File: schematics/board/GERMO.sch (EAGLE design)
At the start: 28 parts

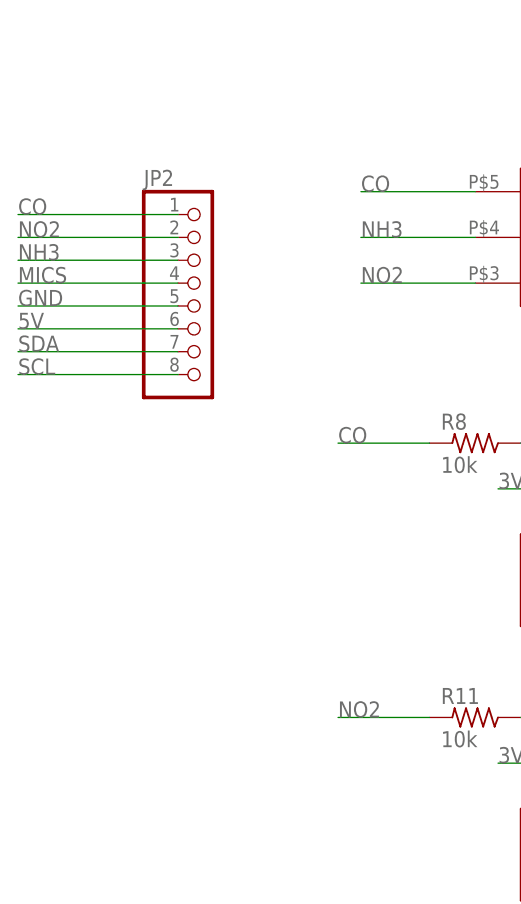
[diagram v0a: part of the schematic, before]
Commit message: сч мипэхъ\
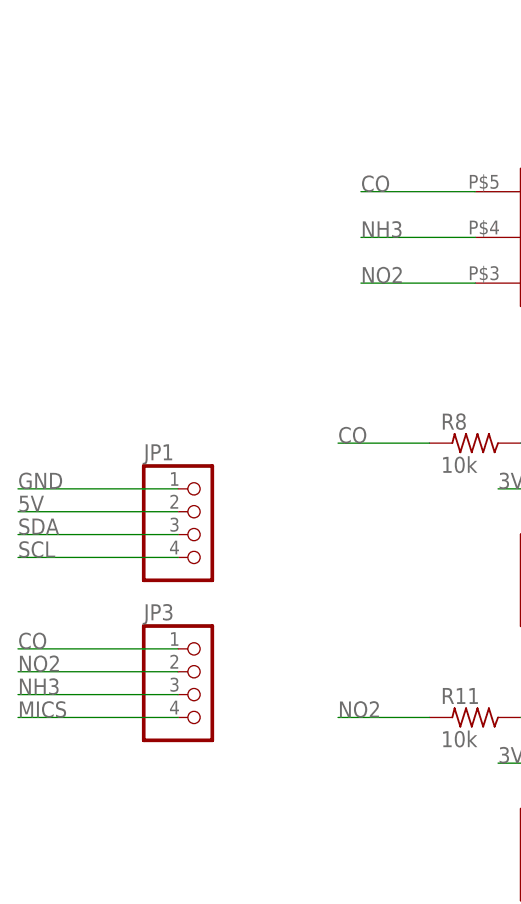
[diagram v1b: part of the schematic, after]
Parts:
- removed JP2: (no value), pinhead:PINHD-1X8
- added JP1, JP3: (no value), pinhead:PINHD-1X4
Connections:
- net 5V: now also JP1.2; no longer JP2.6
- net CO: now also JP3.1; no longer JP2.1
- net GND: now also JP1.1; no longer JP2.5
- net MICS: now also JP3.4; no longer JP2.4
- net NH3: now also JP3.3; no longer JP2.3
- net NO2: now also JP3.2; no longer JP2.2
- net SCL: now also JP1.4; no longer JP2.8
- net SDA: now also JP1.3; no longer JP2.7
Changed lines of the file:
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@@
 <?xml version="1.0" encoding="utf-8"?>
 <!DOCTYPE eagle SYSTEM "eagle.dtd">
-<eagle version="9.4.2">
+<eagle version="9.6.2">
 <drawing>
 <settings>
-<setting alwaysvectorfont="yes"/>
+<setting alwaysvectorfont="no"/>
 <setting verticaltext="up"/>
 </settings>
@@
 </classes>
 <parts>
-<part name="JP2" library="pinhead" library_urn="urn:adsk.eagle:library:325" deviceset="PINHD-1X8" device="" package3d_urn="urn:adsk.eagle:package:22409/2"/>
 <part name="BME280" library="UNKNOWN-2024" deviceset="BME280" device="BME280-PINS-ONLY"/>
 <part name="MICS-6814" library="CanCubeSat" deviceset="MICS-6814" device=""/>
@@
 <part name="U$11" library="UNKNOWN-2024" deviceset="CONNECT_3" device=""/>
 <part name="U$12" library="UNKNOWN-2024" deviceset="CONNECT_3" device=""/>
+<part name="JP1" library="pinhead" library_urn="urn:adsk.eagle:library:325" deviceset="PINHD-1X4" device="" package3d_urn="urn:adsk.eagle:package:22407/2"/>
+<part name="JP3" library="pinhead" library_urn="urn:adsk.eagle:library:325" deviceset="PINHD-1X4" device="" package3d_urn="urn:adsk.eagle:package:22407/2"/>
 </parts>
 <sheets>
@@
 </plain>
 <instances>
-<instance part="JP2" gate="A" x="-101.6" y="43.18" smashed="yes">
-<attribute name="NAME" x="-107.95" y="56.515" size="1.778" layer="95"/>
-<attribute name="VALUE" x="-107.95" y="30.48" size="1.778" layer="96"/>
-</instance>
 <instance part="BME280" gate="G$1" x="86.36" y="20.32" smashed="yes">
 <attribute name="NAME" x="82.296" y="26.416" size="1.27" layer="95"/>
@@
 <instance part="U$12" gate="G$1" x="30.48" y="-12.7" smashed="yes" rot="R270">
 <attribute name="NAME" x="38.1" y="-12.7" size="1.778" layer="95" rot="R270"/>
+</instance>
+<instance part="JP1" gate="A" x="-101.6" y="17.78" smashed="yes">
+<attribute name="NAME" x="-107.95" y="26.035" size="1.778" layer="95"/>
+<attribute name="VALUE" x="-107.95" y="10.16" size="1.778" layer="96"/>
+</instance>
+<instance part="JP3" gate="A" x="-101.6" y="0" smashed="yes">
+<attribute name="NAME" x="-107.95" y="8.255" size="1.778" layer="95"/>
+<attribute name="VALUE" x="-107.95" y="-7.62" size="1.778" layer="96"/>
 </instance>
 </instances>
@@
 <net name="GND" class="0">
 <segment>
-<wire x1="-104.14" y1="43.18" x2="-121.92" y2="43.18" width="0.1524" layer="91"/>
-<label x="-121.92" y="43.18" size="1.778" layer="95"/>
-<pinref part="JP2" gate="A" pin="5"/>
-</segment>
-<segment>
 <wire x1="73.66" y1="17.78" x2="60.96" y2="17.78" width="0.1524" layer="91"/>
 <label x="60.96" y="17.78" size="1.778" layer="95"/>
@@
 <label x="63.5" y="48.26" size="1.778" layer="95"/>
 </segment>
+<segment>
+<wire x1="-104.14" y1="22.86" x2="-121.92" y2="22.86" width="0.1524" layer="91"/>
+<label x="-121.92" y="22.86" size="1.778" layer="95"/>
+<pinref part="JP1" gate="A" pin="1"/>
+</segment>
 </net>
 <net name="5V" class="0">
-<segment>
-<wire x1="-104.14" y1="40.64" x2="-121.92" y2="40.64" width="0.1524" layer="91"/>
-<label x="-121.92" y="40.64" size="1.778" layer="95"/>
-<pinref part="JP2" gate="A" pin="6"/>
-</segment>
 <segment>
 <pinref part="BME280" gate="G$1" pin="VIN"/>
@@
 <label x="83.82" y="58.42" size="1.778" layer="95"/>
 </segment>
+<segment>
+<wire x1="-104.14" y1="20.32" x2="-121.92" y2="20.32" width="0.1524" layer="91"/>
+<label x="-121.92" y="20.32" size="1.778" layer="95"/>
+<pinref part="JP1" gate="A" pin="2"/>
+</segment>
 </net>
 <net name="NO2" class="0">
-<segment>
-<wire x1="-121.92" y1="50.8" x2="-104.14" y2="50.8" width="0.1524" layer="91"/>
-<label x="-121.92" y="50.8" size="1.778" layer="95"/>
-<pinref part="JP2" gate="A" pin="2"/>
-</segment>
 <segment>
 <pinref part="MICS-6814" gate="G$1" pin="NO2"/>
@@
 <label x="-86.36" y="-2.54" size="1.778" layer="95"/>
 </segment>
+<segment>
+<wire x1="-121.92" y1="2.54" x2="-104.14" y2="2.54" width="0.1524" layer="91"/>
+<label x="-121.92" y="2.54" size="1.778" layer="95"/>
+<pinref part="JP3" gate="A" pin="2"/>
+</segment>
 </net>
 <net name="NH3" class="0">
-<segment>
-<wire x1="-104.14" y1="48.26" x2="-121.92" y2="48.26" width="0.1524" layer="91"/>
-<label x="-121.92" y="48.26" size="1.778" layer="95"/>
-<pinref part="JP2" gate="A" pin="3"/>
-</segment>
 <segment>
 <pinref part="MICS-6814" gate="G$1" pin="NH3"/>
@@
 <label x="-12.7" y="27.94" size="1.778" layer="95"/>
 </segment>
+<segment>
+<wire x1="-104.14" y1="0" x2="-121.92" y2="0" width="0.1524" layer="91"/>
+<label x="-121.92" y="0" size="1.778" layer="95"/>
+<pinref part="JP3" gate="A" pin="3"/>
+</segment>
 </net>
 <net name="MICS" class="0">
-<segment>
-<wire x1="-121.92" y1="45.72" x2="-104.14" y2="45.72" width="0.1524" layer="91"/>
-<label x="-121.92" y="45.72" size="1.778" layer="95"/>
-<pinref part="JP2" gate="A" pin="4"/>
-</segment>
 <segment>
 <wire x1="17.78" y1="48.26" x2="5.08" y2="48.26" width="0.1524" layer="91"/>
@@
 <label x="-12.7" y="-2.54" size="1.778" layer="95"/>
 </segment>
+<segment>
+<wire x1="-121.92" y1="-2.54" x2="-104.14" y2="-2.54" width="0.1524" layer="91"/>
+<label x="-121.92" y="-2.54" size="1.778" layer="95"/>
+<pinref part="JP3" gate="A" pin="4"/>
+</segment>
 </net>
 <net name="SDA" class="0">
-<segment>
-<wire x1="-104.14" y1="38.1" x2="-121.92" y2="38.1" width="0.1524" layer="91"/>
-<label x="-121.92" y="38.1" size="1.778" layer="95"/>
-<pinref part="JP2" gate="A" pin="7"/>
-</segment>
 <segment>
 <wire x1="99.06" y1="17.78" x2="114.3" y2="17.78" width="0.1524" layer="91"/>
@@
 <label x="83.82" y="50.8" size="1.778" layer="95"/>
 </segment>
+<segment>
+<wire x1="-104.14" y1="17.78" x2="-121.92" y2="17.78" width="0.1524" layer="91"/>
+<label x="-121.92" y="17.78" size="1.778" layer="95"/>
+<pinref part="JP1" gate="A" pin="3"/>
+</segment>
 </net>
 <net name="SCL" class="0">
-<segment>
-<wire x1="-104.14" y1="35.56" x2="-121.92" y2="35.56" width="0.1524" layer="91"/>
-<label x="-121.92" y="35.56" size="1.778" layer="95"/>
-<pinref part="JP2" gate="A" pin="8"/>
-</segment>
 <segment>
 <wire x1="99.06" y1="22.86" x2="114.3" y2="22.86" width="0.1524" layer="91"/>
@@
 <label x="83.82" y="53.34" size="1.778" layer="95"/>
 </segment>
+<segment>
+<wire x1="-104.14" y1="15.24" x2="-121.92" y2="15.24" width="0.1524" layer="91"/>
+<label x="-121.92" y="15.24" size="1.778" layer="95"/>
+<pinref part="JP1" gate="A" pin="4"/>
+</segment>
 </net>
 <net name="CO" class="0">
@@
 </segment>
 <segment>
-<wire x1="-104.14" y1="53.34" x2="-121.92" y2="53.34" width="0.1524" layer="91"/>
-<label x="-121.92" y="53.34" size="1.778" layer="95"/>
-<pinref part="JP2" gate="A" pin="1"/>
-</segment>
-<segment>
 <pinref part="R8" gate="G$1" pin="2"/>
 <wire x1="-76.2" y1="27.94" x2="-86.36" y2="27.94" width="0.1524" layer="91"/>
 <label x="-86.36" y="27.94" size="1.778" layer="95"/>
 </segment>
-</net>
+<segment>
+<wire x1="-104.14" y1="5.08" x2="-121.92" y2="5.08" width="0.1524" layer="91"/>
+<label x="-121.92" y="5.08" size="1.778" layer="95"/>
+<pinref part="JP3" gate="A" pin="1"/>
+</segment>
+</net>
